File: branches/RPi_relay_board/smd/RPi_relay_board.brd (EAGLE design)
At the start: 81 x 88.3 mm, 48 parts, among them IC1 LM340S-05, K1 351, K2 351, T1 ZXTN2020F, T2 ZXTN2020F, T3 ZXTN2020F, U1 MAX232SOIC16

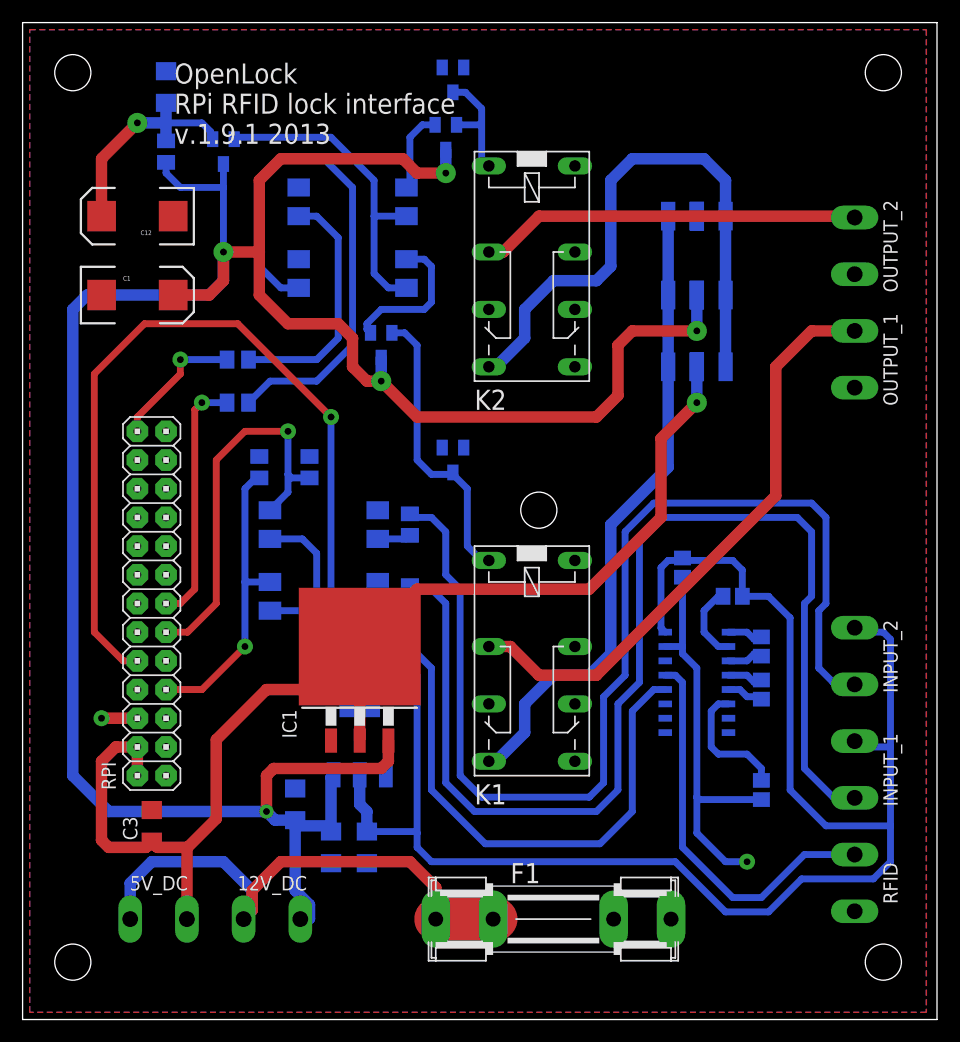
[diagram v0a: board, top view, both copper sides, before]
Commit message: Version 2.0-series of pcb
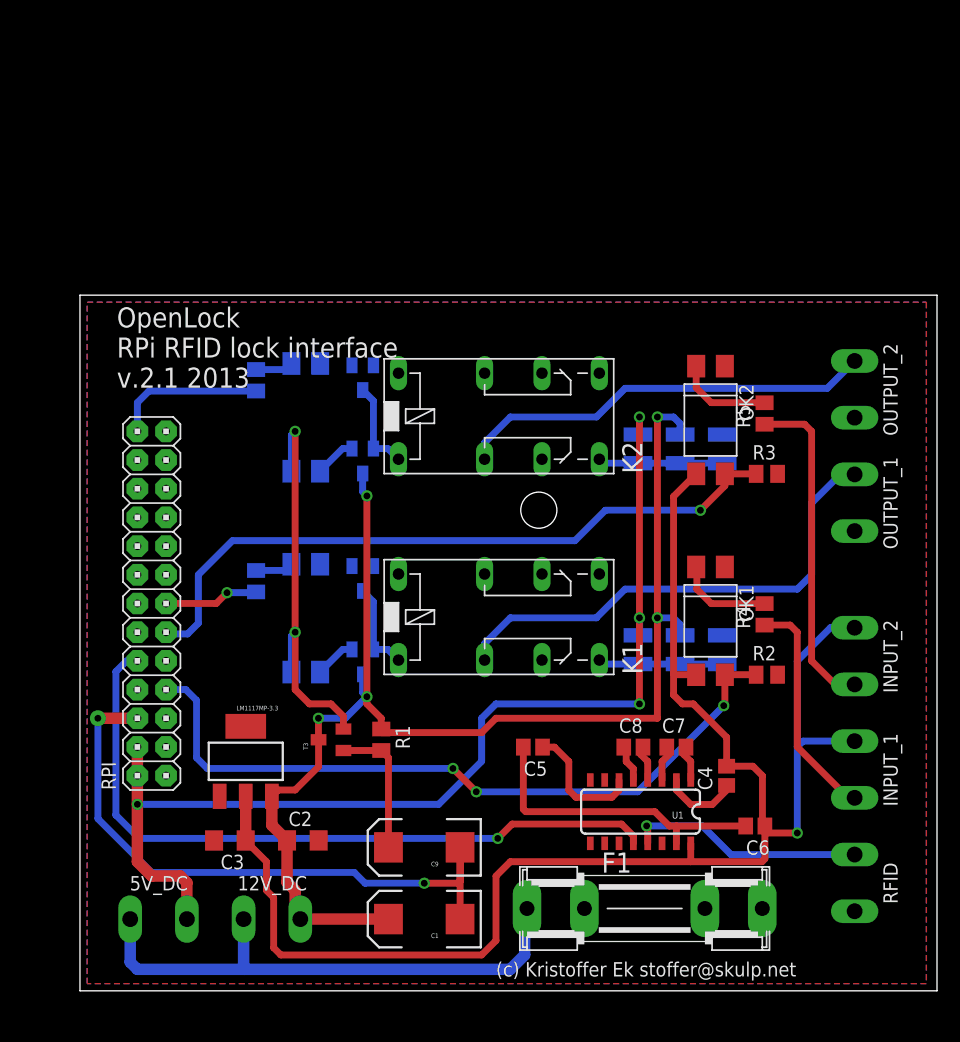
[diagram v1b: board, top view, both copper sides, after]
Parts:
- removed C10: 100nF, rcl:C2012
- removed C11: 10uF, rcl:C3216
- removed C12: 330nF, SparkFun:EIA7343
- removed IC1: LM340S-05, LM1084IS:TO263-3
- C4: value 330nF -> 100nF; device rcl:C3216 -> rcl:C2012
- C5: device rcl:C3216 -> rcl:C2012
- C9: value 100nF -> 330nF; device rcl:C2012 -> SparkFun:EIA7343
- moved C1 60.8 mm to (39.4, 0.00), turned to 180 degrees
- moved R1 55.4 mm to (35.6, 15.9), flipped to the top, turned to 270 degrees
- moved T3 52.9 mm to (31.1, 15.9), flipped to the top, turned to 90 degrees
- moved R2 48.5 mm to (69.7, 21.6), flipped to the top, turned to 0 degrees
- moved R3 40.5 mm to (69.7, 39.4), flipped to the top, turned to 0 degrees
- moved SJ1_GND 38.5 mm to (65.8, 23.8), turned to 90 degrees
- moved C4 35.6 mm to (66.1, 12.7), flipped to the top, turned to 90 degrees
- moved OK2 35.5 mm to (64.7, 44.2), flipped to the top, turned to 180 degrees
- moved C9 34.7 mm to (39.4, 6.35), flipped to the top, turned to 180 degrees
- moved OK1 34.3 mm to (64.7, 26.4), flipped to the top, turned to 180 degrees
- moved R5 32.9 mm to (69.5, 44.8), flipped to the top, turned to 90 degrees
- moved R4 31.4 mm to (69.5, 27.0), flipped to the top, turned to 90 degrees
- moved SJ1_12V 31.4 mm to (62.0, 23.8), turned to 90 degrees
- moved OK3 30.8 mm to (28.9, 26.6), turned to 180 degrees
- moved T2 29.6 mm to (33.9, 40.6)
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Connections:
- net +12V: no longer C4.1, IC1.3
- net +5V: no longer C3.1, IC1.2, IC1.TAB
- net 3.3V: now also C3.1, C4.2, C6.1; no longer C5.1, C6.2, C8.1
- net GND: now also C6.2, C9.C; no longer C11.2, C12.C, C4.2, C7.2, C8.2, IC1.1
- net N$10: now also C9.A; no longer C11.1, C12.A
- net N$13: now also C7.2; no longer C9.2
- net N$31: now also C8.2; no longer C10.2
- net N$32: now also C7.1; no longer C9.1
- net N$35: now also C8.1; no longer C10.1
- net N$36: now also C4.1; no longer C6.1
- net N$37: now also C5.1; no longer C7.1
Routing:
- net +12V: track 225.0 -> 118.3 mm
- net N$3: track 103.1 -> 20.3 mm
- net N$5: track 99.8 -> 29.8 mm
- net N$15: track 127.5 -> 63.3 mm
- net N$20: track 57.1 -> 11.0 mm
- net GND: track 39.2 -> 83.6 mm
- net N$51: track 47.3 -> 3.35 mm
- net N$18: track 51.8 -> 11.0 mm
- net N$4: track 26.9 -> 64.8 mm, vias 1 -> 3
- net 3.3V: track 171.1 -> 138.6 mm, vias 0 -> 1
- net N$1: track 35.3 -> 61.3 mm
- net N$19: track 21.9 -> 3.35 mm
- net N$12: track 26.1 -> 8.18 mm
- net N$16: track 35.1 -> 21.1 mm, vias 0 -> 1
- net N$44: track 22.1 -> 8.39 mm
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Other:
- board size 81 x 88.3 mm -> 75.9 x 61.6 mm
- board text added: "(c) Kristoffer Ek stoffer@skulp.net"
- board text added: "12V"
- board text added: "5V"
- board text added: "GND"
- board text added: "INPUT 1"
- board text added: "INPUT 2"
- board text added: "OpenLock RPi RFID lock interface v.2.1 2013"
- board text added: "RELAY 1"
- board text added: "RELAY 2"
- board text added: "RFID"
- board text removed: "OUTPUT 1"
- board text removed: "OUTPUT 2"
- board text removed: "OpenLock RPi RFID lock interface v.1.9.1 2013"
